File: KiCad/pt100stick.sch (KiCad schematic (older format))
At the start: 10 parts, among them U1 MAX31865ATP_

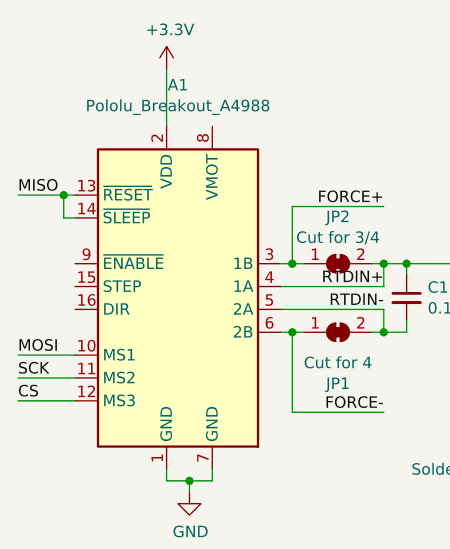
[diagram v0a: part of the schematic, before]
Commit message: Hopefully stable release :D
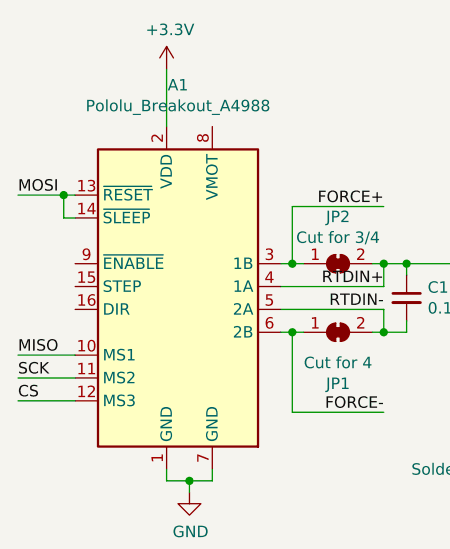
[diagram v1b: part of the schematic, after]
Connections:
- net MISO: now also A1.10 (MS1); no longer A1.13 (~RESET), A1.14 (~SLEEP)
- net MOSI: now also A1.13 (~RESET), A1.14 (~SLEEP); no longer A1.10 (MS1)
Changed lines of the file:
@@
 Wire Wire Line
 	1500 2350 1250 2350
+Text Label 1250 1650 0    50   ~ 0
+MOSI
 Text Label 1250 2350 0    50   ~ 0
-MOSI
-Text Label 1250 1650 0    50   ~ 0
 MISO
 Text Label 1250 2550 0    50   ~ 0

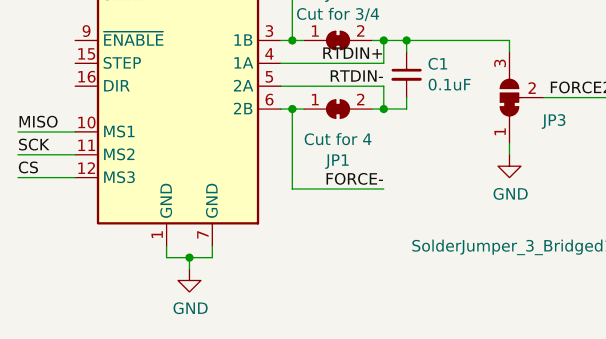
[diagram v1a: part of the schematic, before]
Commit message: Quick fixes
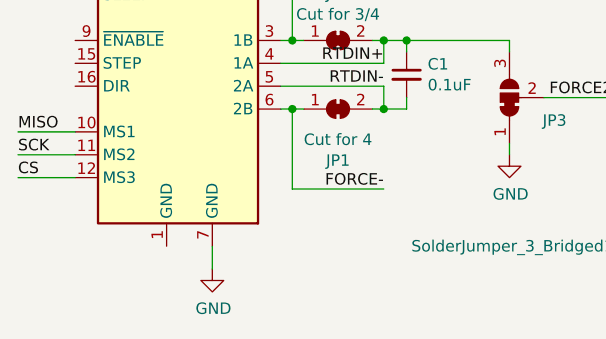
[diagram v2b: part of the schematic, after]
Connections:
- net GND: no longer A1.1 (GND)
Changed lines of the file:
@@
 Comment4 ""
 $EndDescr
-$Comp
-L PT100stick:Pololu_Breakout_A4988 A1
-U 1 1 5EB9E565
-P 1900 2050
-F 0 "A1" H 1950 2931 50  0000 C CNN
-F 1 "Pololu_Breakout_A4988" H 1950 2840 50  0000 C CNN
-F 2 "PT100Stick:Pololu_Breakout-16_15.2x20.3mm" H 2175 1300 50  0001 L CNN
-F 3 "https://www.pololu.com/product/2980/pictures" H 2000 1750 50  0001 C CNN
-	1    1900 2050
-	1    0    0    -1
-$EndComp
 Wire Wire Line
 	1500 2550 1250 2550
@@
 L PT100stick:GND #PWR0101
 U 1 1 5EBA0B0B
-P 2000 2950
-F 0 "#PWR0101" H 2000 2700 50  0001 C CNN
-F 1 "GND" H 2005 2777 50  0000 C CNN
-F 2 "" H 2000 2950 50  0001 C CNN
-F 3 "" H 2000 2950 50  0001 C CNN
-	1    2000 2950
-	1    0    0    -1
-$EndComp
-Wire Wire Line
-	1900 2850 1900 2900
-Wire Wire Line
-	2100 2900 2100 2850
-Wire Wire Line
-	1900 2900 2000 2900
-Wire Wire Line
-	2000 2950 2000 2900
-Connection ~ 2000 2900
-Wire Wire Line
-	2000 2900 2100 2900
+P 2100 2950
+F 0 "#PWR0101" H 2100 2700 50  0001 C CNN
+F 1 "GND" H 2105 2777 50  0000 C CNN
+F 2 "" H 2100 2950 50  0001 C CNN
+F 3 "" H 2100 2950 50  0001 C CNN
+	1    2100 2950
+	1    0    0    -1
+$EndComp
 $Comp
 L PT100stick:+3.3V #PWR0102
@@
 	1    0    0    -1
 $EndComp
+$Comp
+L PT100stick:Pololu_Breakout_A4988 A1
+U 1 1 5EB9E565
+P 1900 2050
+F 0 "A1" H 1950 2931 50  0000 C CNN
+F 1 "Pololu_Breakout_A4988" H 1950 2840 50  0000 C CNN
+F 2 "PT100Stick:Pololu_Breakout-16_15.2x20.3mm" H 2175 1300 50  0001 L CNN
+F 3 "https://www.pololu.com/product/2980/pictures" H 2000 1750 50  0001 C CNN
+	1    1900 2050
+	1    0    0    -1
+$EndComp
+Wire Wire Line
+	2100 2850 2100 2950
 $EndSCHEMATC
